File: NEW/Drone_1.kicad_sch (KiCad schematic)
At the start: 28 parts, among them J1 ESP-32_DevkitC, J2 Conn_01x08_Pin, U1 Rasberry Pi 0W, U3 GY-NEO6MV2, U4 BME280, U5 HMC5883L, U6 mp1584, U7 mp1584, U8 Flysky fs-a8s

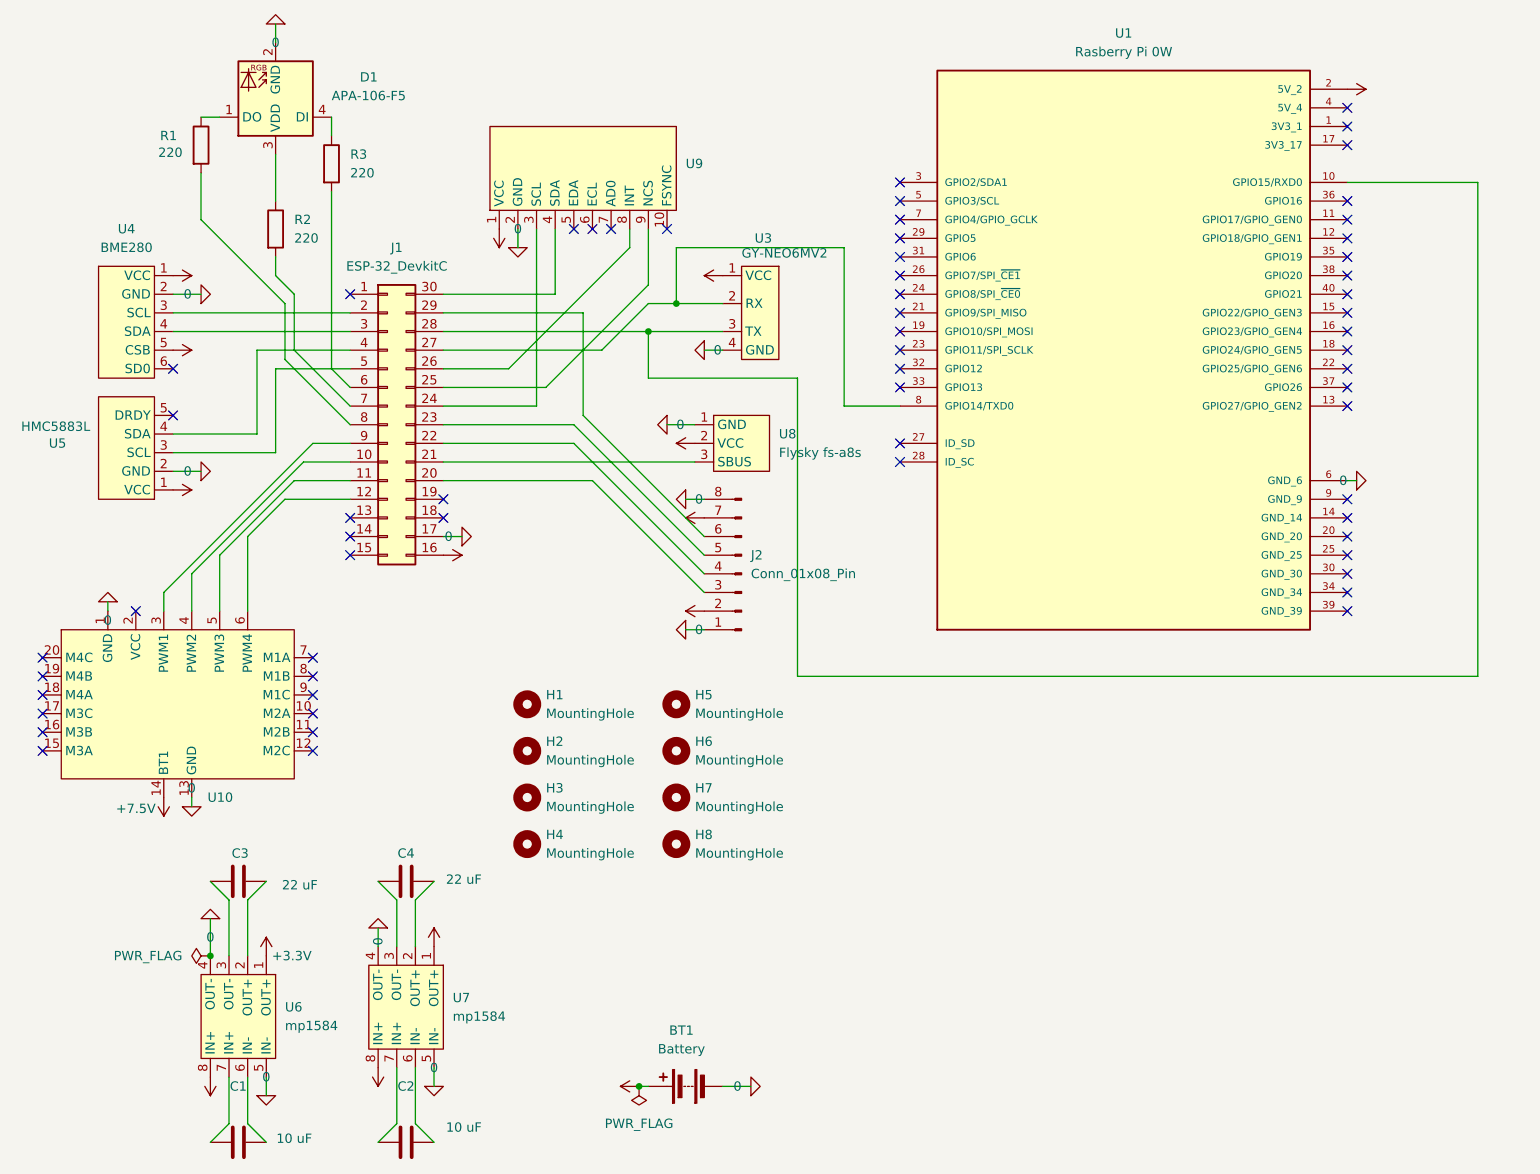
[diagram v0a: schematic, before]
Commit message: welcome
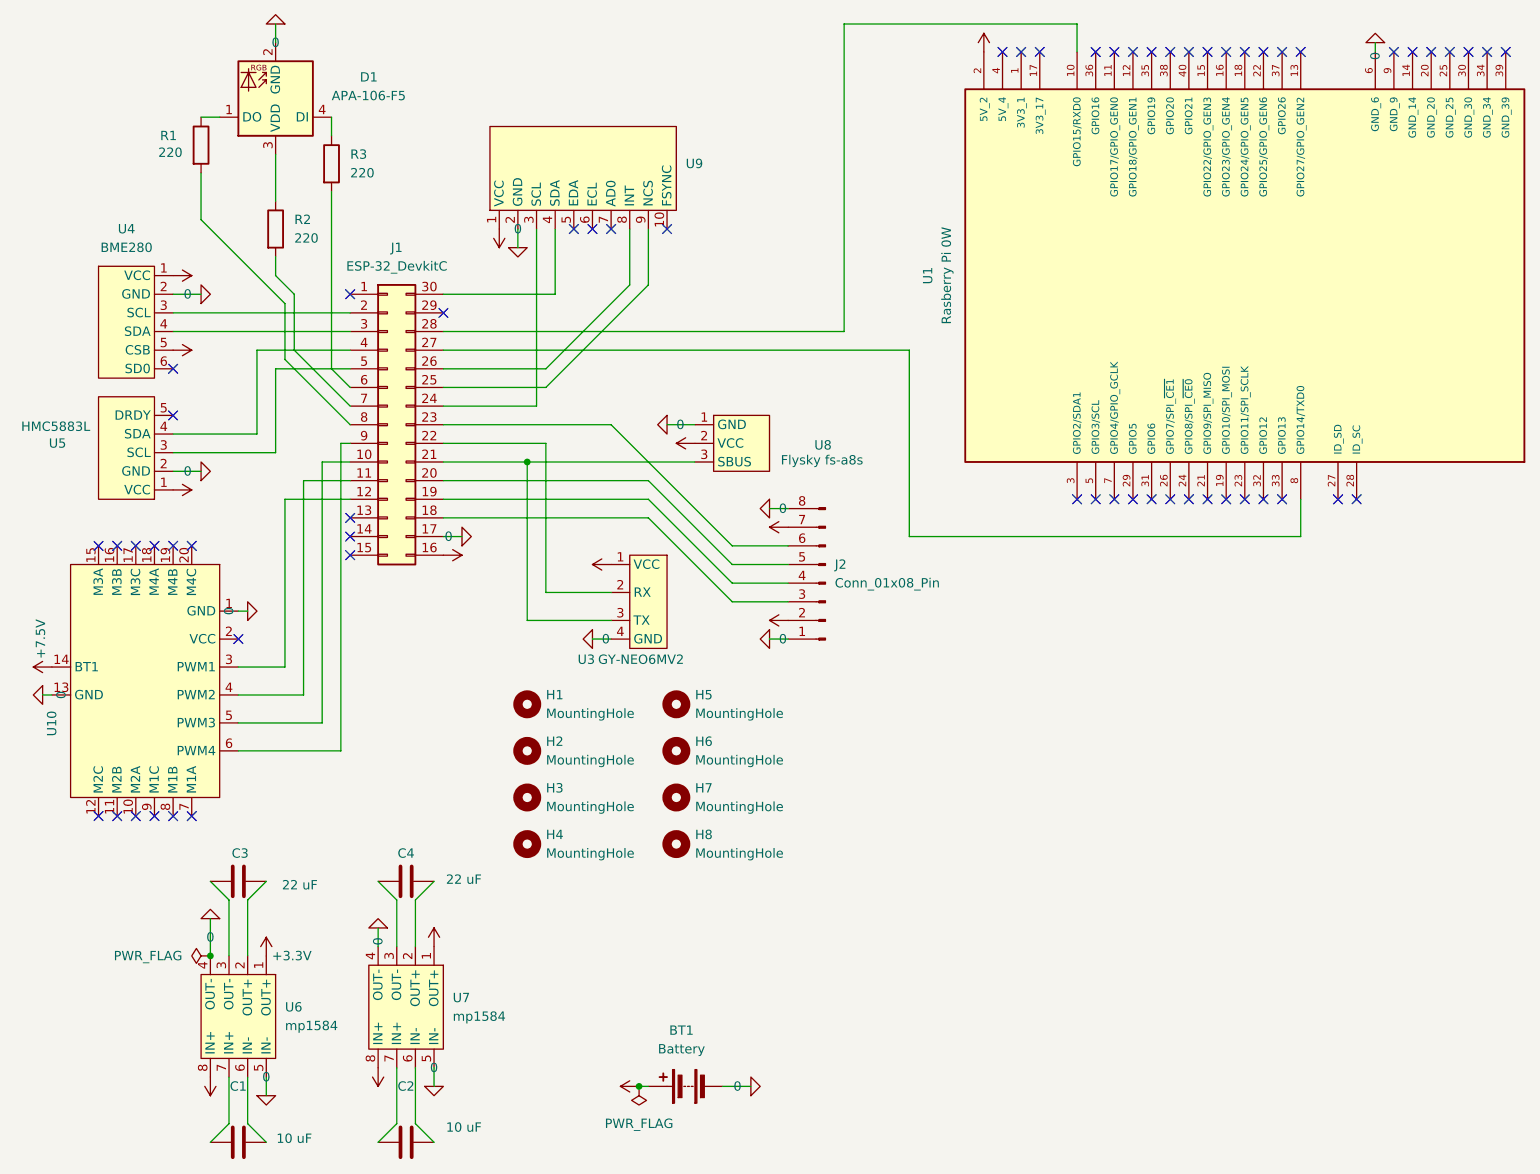
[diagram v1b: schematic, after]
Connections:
- net +3.3V: now also J2.2 (Pin_2); no longer J2.7 (Pin_7)
- net +5V: now also J2.7 (Pin_7); no longer J2.2 (Pin_2)
- net at J2.3 (Pin_3): now also J1.18 (Pin_18); no longer J1.20 (Pin_20)
- net at J2.4 (Pin_4): now also J1.19 (Pin_19); no longer J1.22 (Pin_22)
- net at J2.5 (Pin_5): now also J1.20 (Pin_20); no longer J1.23 (Pin_23)
- net at J2.6 (Pin_6): now also J1.23 (Pin_23); no longer J1.29 (Pin_29)
- net at J1.10 (Pin_10): now also U10.5 (PWM3); no longer U10.4 (PWM2)
- net at J1.11 (Pin_11): now also U10.4 (PWM2); no longer U10.5 (PWM3)
- net at J1.12 (Pin_12): now also U10.3 (PWM1); no longer U10.6 (PWM4)
- net at J1.21 (Pin_21), U8.3 (SBUS): now also U3.3 (TX)
- net at J1.27 (Pin_27), U1.8 (GPIO14/TXD0): no longer U3.2 (RX)
- net at J1.28 (Pin_28), U1.10 (GPIO15/RXD0): no longer U3.3 (TX)
- net at J1.9 (Pin_9): now also U10.6 (PWM4); no longer U10.3 (PWM1)
- new net: J1.22 (Pin_22), U3.2 (RX)
- no-connect marks 61 -> 60
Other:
- moved on the sheet: J2, U1, U10, U3

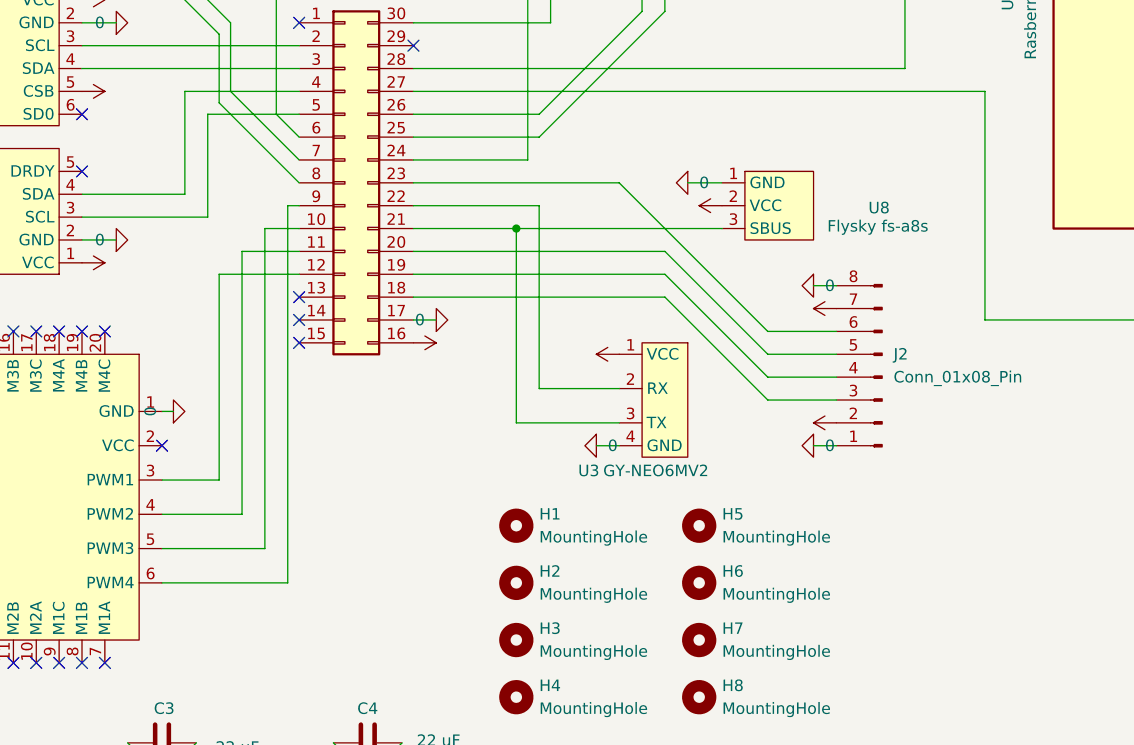
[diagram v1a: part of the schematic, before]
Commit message: welcome
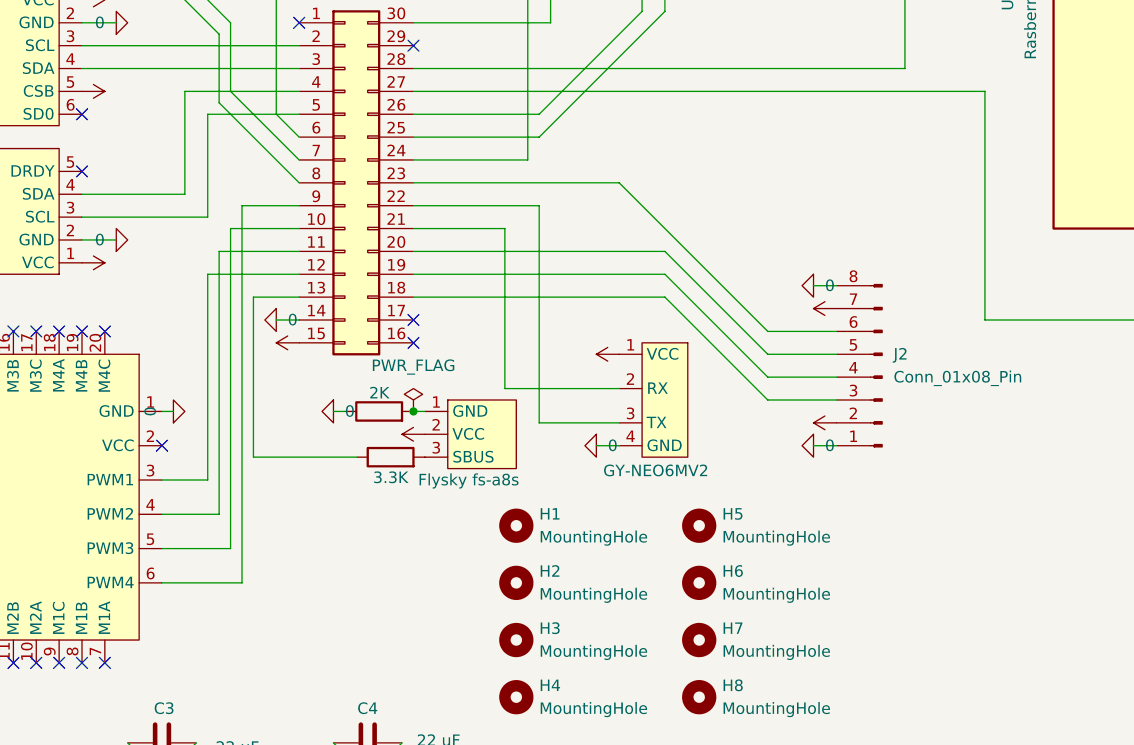
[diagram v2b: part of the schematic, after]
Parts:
- added R4: 3.3K, Resistor_THT:R_Axial_DIN0204_L3.6mm_D1.6mm_P5.08mm_Horizontal, symbol Device:R
- added R5: 2K, Resistor_THT:R_Axial_DIN0204_L3.6mm_D1.6mm_P5.08mm_Horizontal, symbol Device:R
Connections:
- net +3.3V: now also J1.15 (Pin_15); no longer J1.16 (Pin_16)
- net 0: now also J1.14 (Pin_14), R5.1; no longer J1.17 (Pin_17), U8.1 (GND)
- net at J1.13 (Pin_13): now also R4.1
- net at U3.2 (RX): now also J1.21 (Pin_21); no longer J1.22 (Pin_22)
- new net: R5.2, U8.1 (GND)
- new net: J1.22 (Pin_22), U3.3 (TX)
- new net: R4.2, U8.3 (SBUS)
- no-connect marks 60 -> 59
